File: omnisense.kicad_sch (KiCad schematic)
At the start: 17 parts, among them J2 USB_C_Receptacle_USB2.0_16P, U1 ESP32-S3-WROOM-1, U3 TLV76133DCY

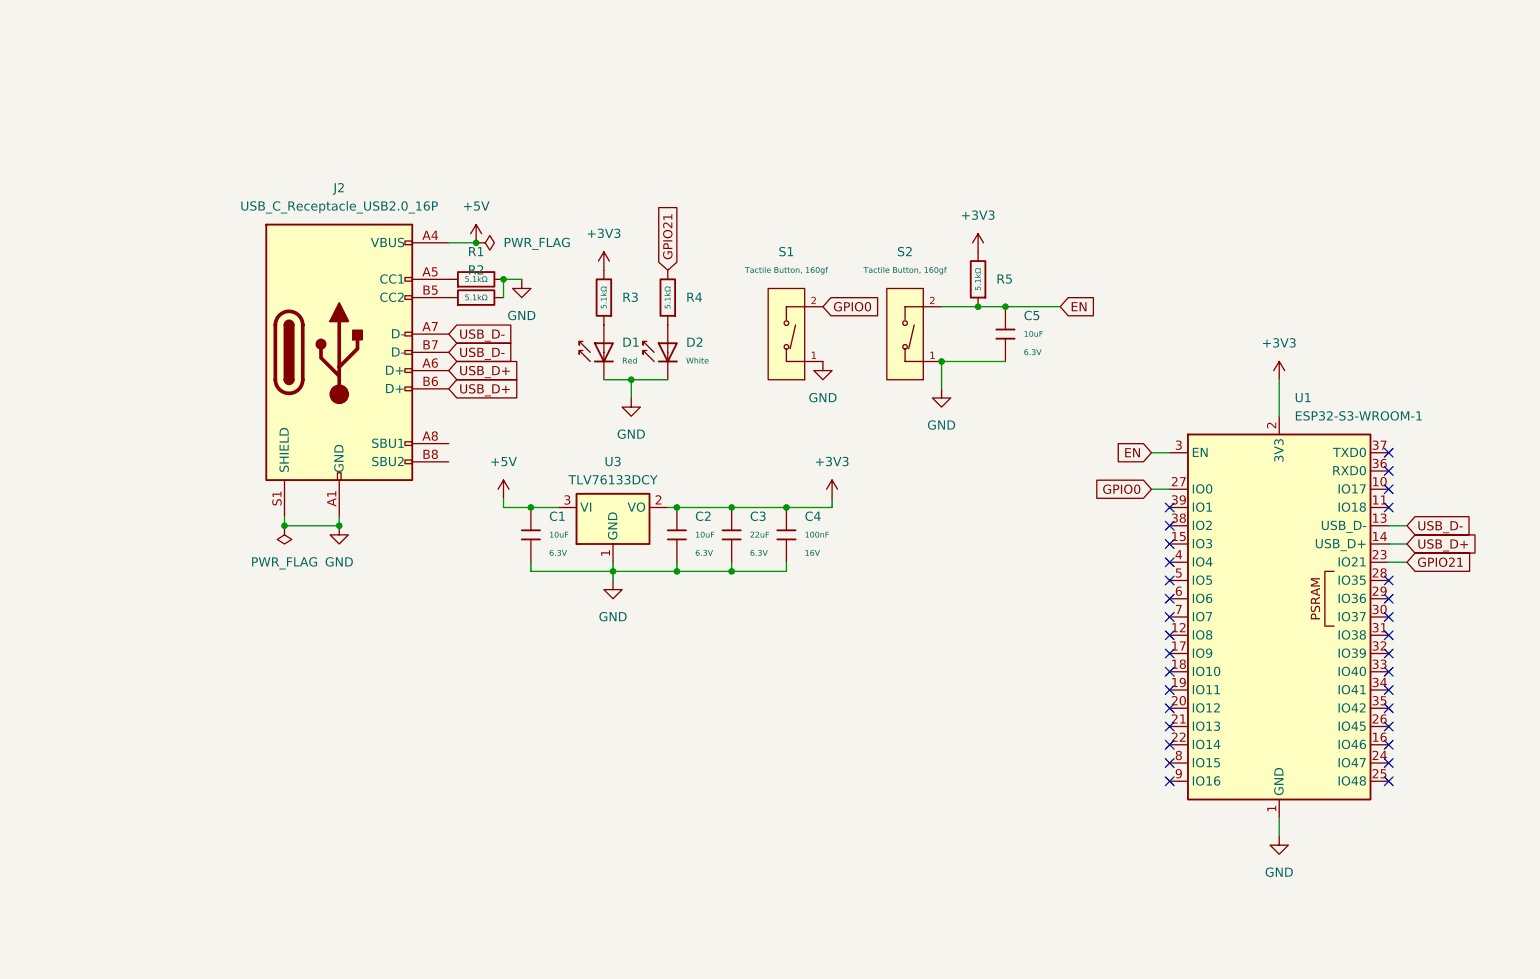
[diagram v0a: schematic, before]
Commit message: lgtm
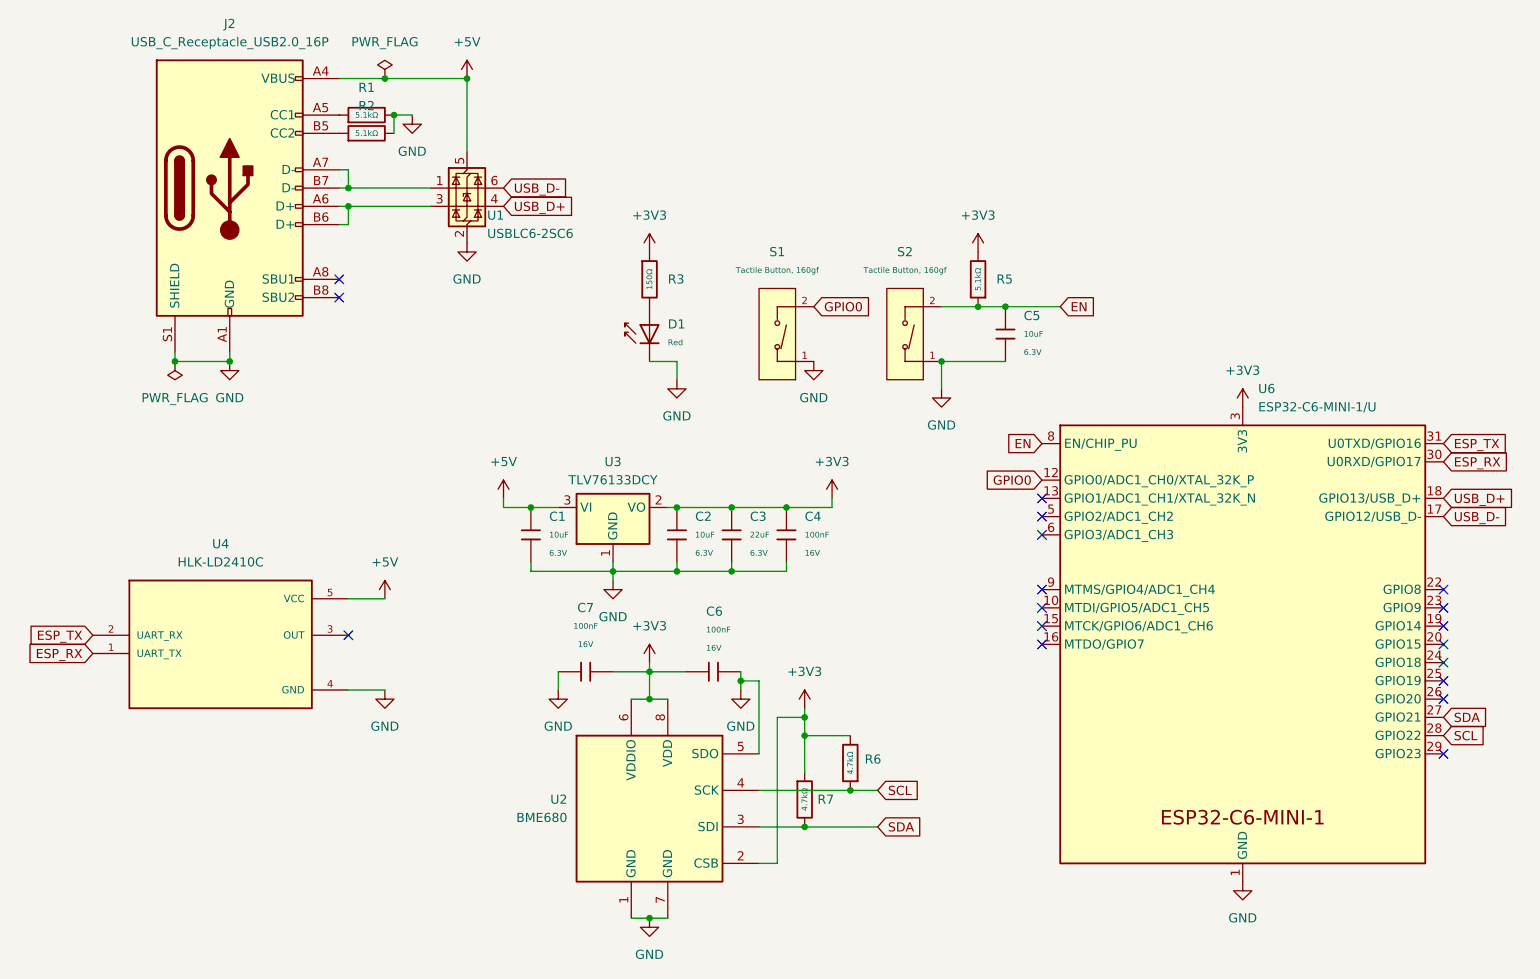
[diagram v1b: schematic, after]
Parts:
- removed D1: Red, PCM_JLCPCB:D_0805, symbol PCM_JLCPCB-Diodes:LED,0805,Red
- removed D2: White, PCM_JLCPCB:D_0805, symbol PCM_JLCPCB-Diodes:LED,0805,White
- removed R3, R4: 5.1kΩ, PCM_JLCPCB:R_0402, symbol PCM_JLCPCB-Resistors:0402,5.1kΩ
- removed U1: ESP32-S3-WROOM-1, RF_Module:ESP32-S3-WROOM-1, symbol RF_Module:ESP32-S3-WROOM-1
- added C6, C7: 100nF, PCM_JLCPCB:C_0402, symbol PCM_JLCPCB-Capacitors:0402,100nF
- added D1: Red, PCM_JLCPCB:D_0603, symbol PCM_JLCPCB-Diodes:LED,0603,Red
- added R3: 150Ω, PCM_JLCPCB:R_0402, symbol PCM_JLCPCB-Resistors:0402,150Ω
- added R6, R7: 4.7kΩ, PCM_JLCPCB:R_0402, symbol PCM_JLCPCB-Resistors:0402,4.7kΩ
- added U1: USBLC6-2SC6, Package_TO_SOT_SMD:SOT-23-6, symbol Power_Protection:USBLC6-2SC6
- added U2: BME680, Package_LGA:Bosch_LGA-8_3x3mm_P0.8mm_ClockwisePinNumbering, symbol Sensor:BME680
- added U4: HLK-LD2410C, HLK-LD2410C:MODULE_HLK-LD2410C, symbol HLK-LD2410C:HLK-LD2410C
- added U6: ESP32-C6-MINI-1/U, PCM_Espressif:ESP32-C6-MINI-1, symbol PCM_Espressif:ESP32-C6-MINI-1/U
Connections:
- net +3V3: now also C6.1, C7.1, R3.1, R6.2, R7.1, U2.2 (CSB), U2.6 (VDDIO), U2.8 (VDD), U6.3 (3V3)
- net +5V: now also U1.5 (VBUS), U4.5 (VCC)
- net EN: now also U6.8 (EN/CHIP_PU)
- net GND: now also C6.2, C7.2, D1.1, U1.2 (GND), U2.1 (GND), U2.5 (SDO), U2.7 (GND), U4.4 (GND), U6.1 (GND), U6.11 (GND), U6.14 (GND), U6.2 (GND), U6.36 (GND), U6.37 (GND), U6.38 (GND), U6.39 (GND), U6.40 (GND), U6.41 (GND), U6.42 (GND), U6.43 (GND), U6.44 (GND), U6.45 (GND), U6.46 (GND), U6.47 (GND), U6.48 (GND), U6.49 (GND), U6.50 (GND), U6.51 (GND), U6.52 (GND), U6.53 (GND)
- net GPIO0: now also U6.12 (GPIO0/ADC1_CH0/XTAL_32K_P)
- net USB_D+: now also U1.4 (I/O2), U6.18 (GPIO13/USB_D+); no longer J2.A6 (D+), J2.B6 (D+)
- net USB_D-: now also U1.6 (I/O1), U6.17 (GPIO12/USB_D-); no longer J2.A7 (D-), J2.B7 (D-)
- new net: D1.2, R3.2
- new net: J2.A6 (D+), J2.B6 (D+), U1.3 (I/O2)
- new net: J2.A7 (D-), J2.B7 (D-), U1.1 (I/O1)
- new net ESP_RX: U4.1 (UART_TX), U6.30 (U0RXD/GPIO17)
- new net ESP_TX: U4.2 (UART_RX), U6.31 (U0TXD/GPIO16)
- new net SCL: R6.1, U2.4 (SCK), U6.28 (GPIO22)
- new net SDA: R7.2, U2.3 (SDI), U6.27 (GPIO21)
- no-connect marks 32 -> 18
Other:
- moved on the sheet: J2, R1, R2, S1
